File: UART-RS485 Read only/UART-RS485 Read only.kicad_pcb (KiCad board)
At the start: 2 copper layers, 45 x 25 mm, 22 parts, among them J1 Conn_01x02_Socket, J2 UART, J3 RS485, U1 MIC5504-3.3YM5, U2 MAX3485

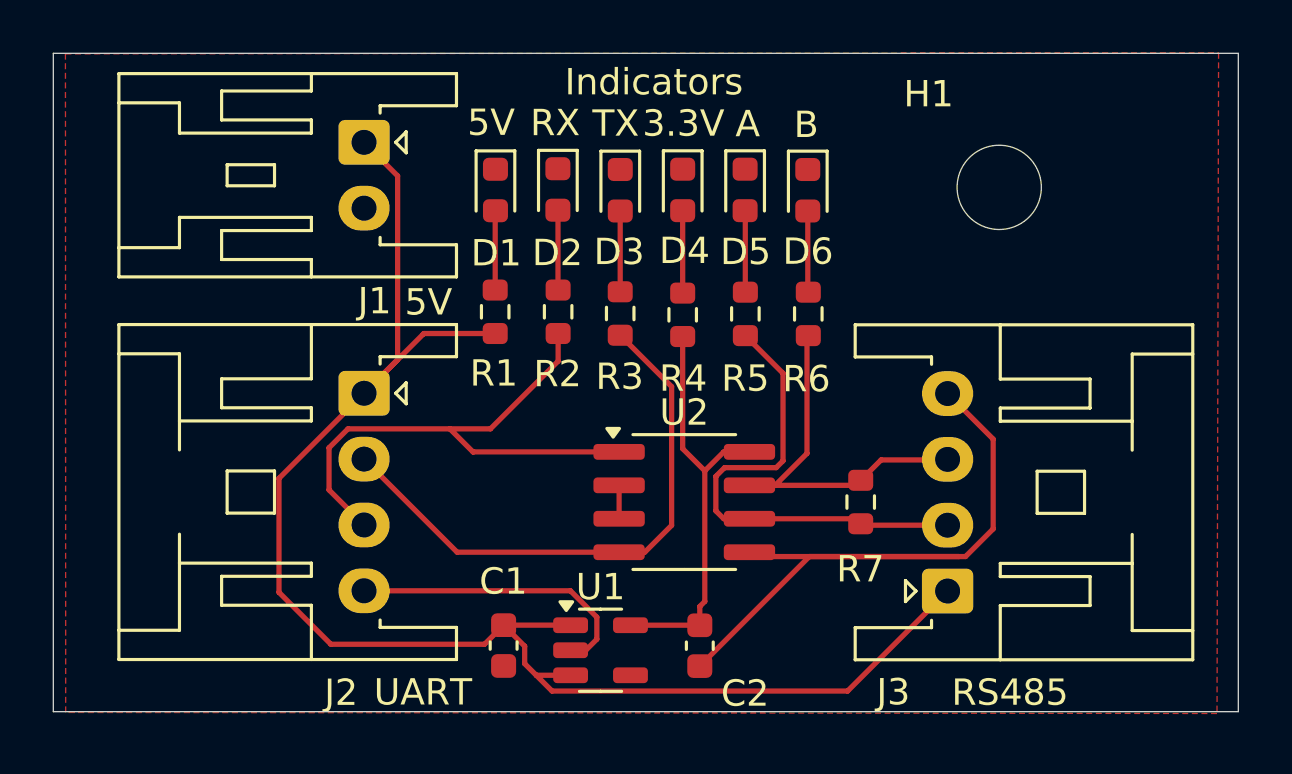
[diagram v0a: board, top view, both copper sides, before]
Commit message: Add files via upload
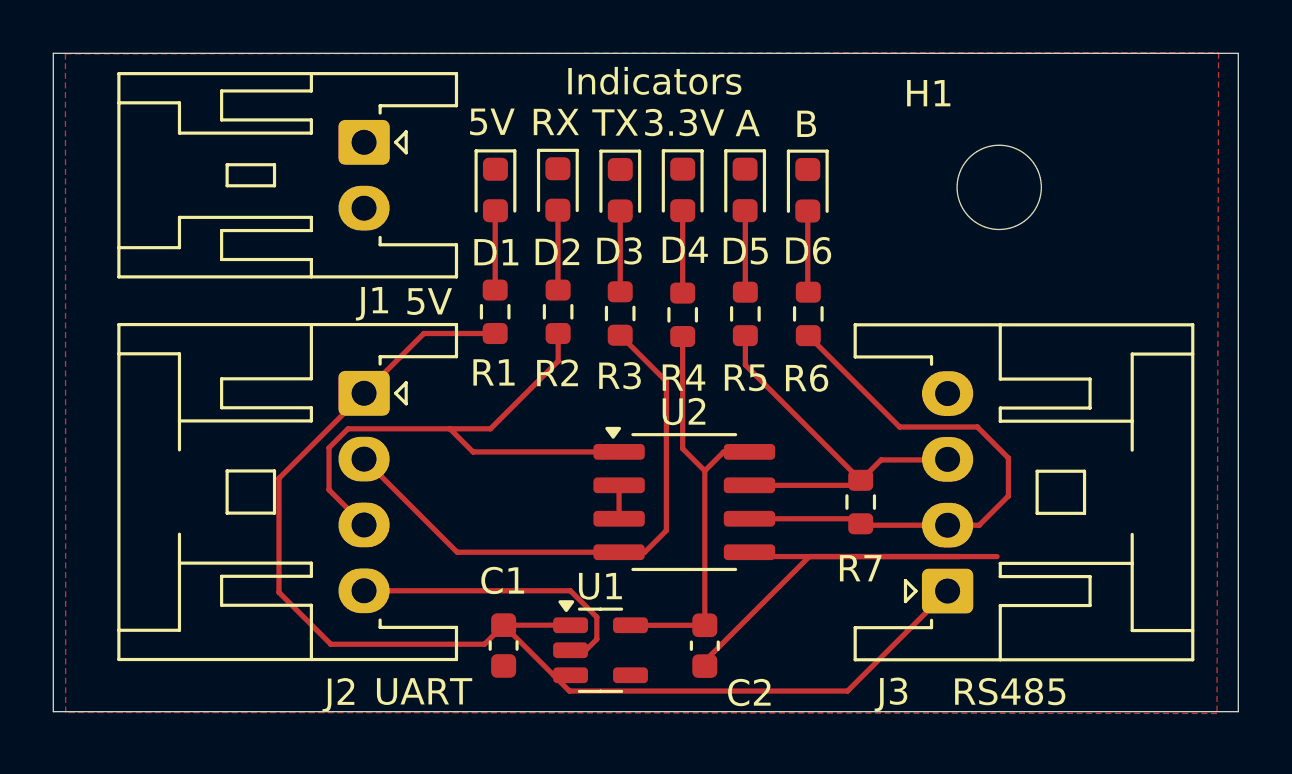
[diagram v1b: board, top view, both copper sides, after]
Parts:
- moved C2 0.19 mm to (160.8, 111.3)
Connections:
- J1 pad 1: +5V -> Net-(J1-Pin_1)
- J1 pad 2: GND -> unconnected-(J1-Pin_2-Pad2)
- R5 pad 1: /A -> /B
- R6 pad 1: /B -> /A
- U2 pad 2: Net-(U2-DE) -> Net-(J1-Pin_1)
- U2 pad 3: Net-(U2-DE) -> Net-(J1-Pin_1)
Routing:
- net +5V: track 58.8 -> 47.1 mm
- net GND: track 38.4 -> 32.3 mm
- net /A: track 18.6 -> 21.5 mm
- net Net-(U2-DE): track 1.27 -> 0.00 mm
- net Net-(J1-Pin_1): track 0.00 -> 1.27 mm
